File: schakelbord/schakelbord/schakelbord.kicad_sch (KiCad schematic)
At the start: 101 parts, among them J1 Rookmachine, J12 I/O nano, J15 Relais 7&8, J16 Alalog i/o, J17 Extra 1-4, J18 Extra 5-8, J19 Relais 5&6, J20 Relais 3&4, J21 Relais 1&2, J3 Power, J4 mosfets, K10 SANYOU_SRD_Form_C, K3 SANYOU_SRD_Form_C, K4 SANYOU_SRD_Form_C, K5 SANYOU_SRD_Form_C, K6 SANYOU_SRD_Form_C, K7 SANYOU_SRD_Form_C, K8 SANYOU_SRD_Form_C, K9 SANYOU_SRD_Form_C, Q1 BC337, Q10 BC337, Q11 BC337, Q12 BC337, Q13 BC337, Q14 BC337, Q15 IRLZ44N, Q2 IRLZ44N, Q3 IRLZ44N, Q5 BC337, Q6 BC337, Q9 BC337, U1 MCP23017x-x-SP

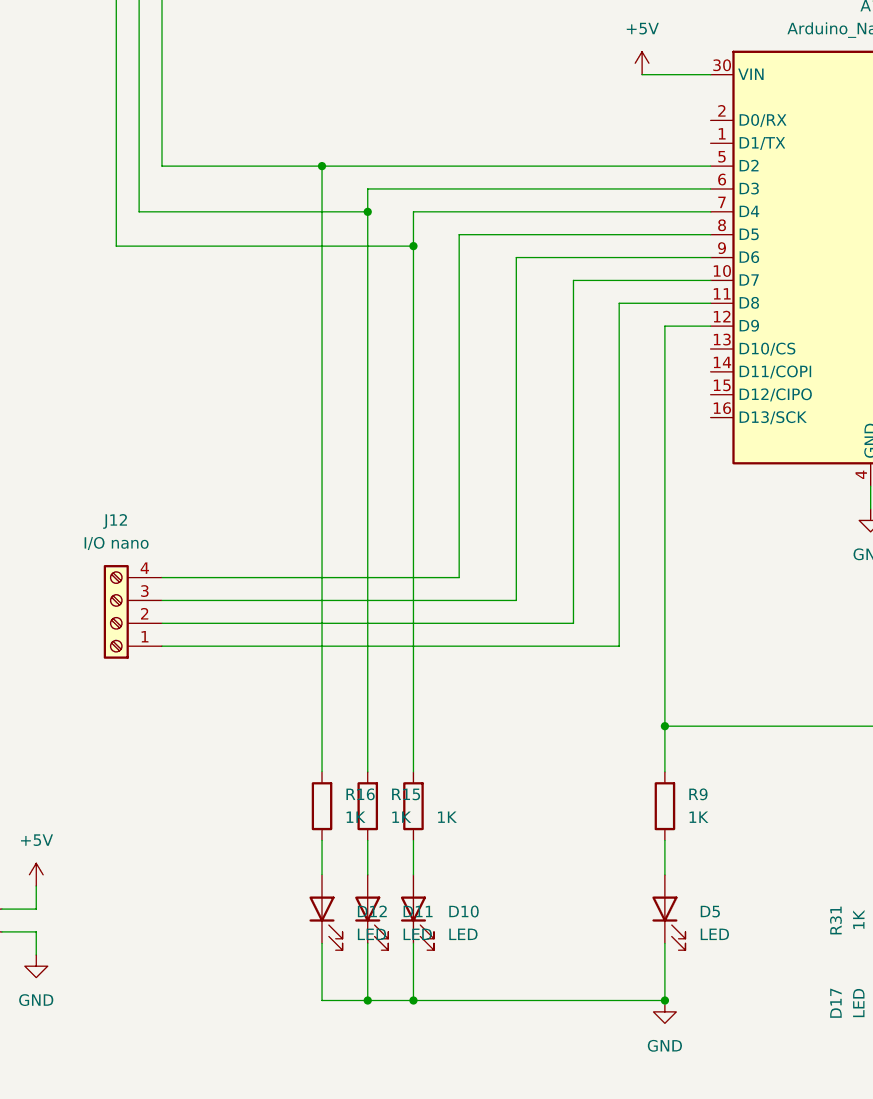
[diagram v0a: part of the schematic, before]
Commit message: pcb update
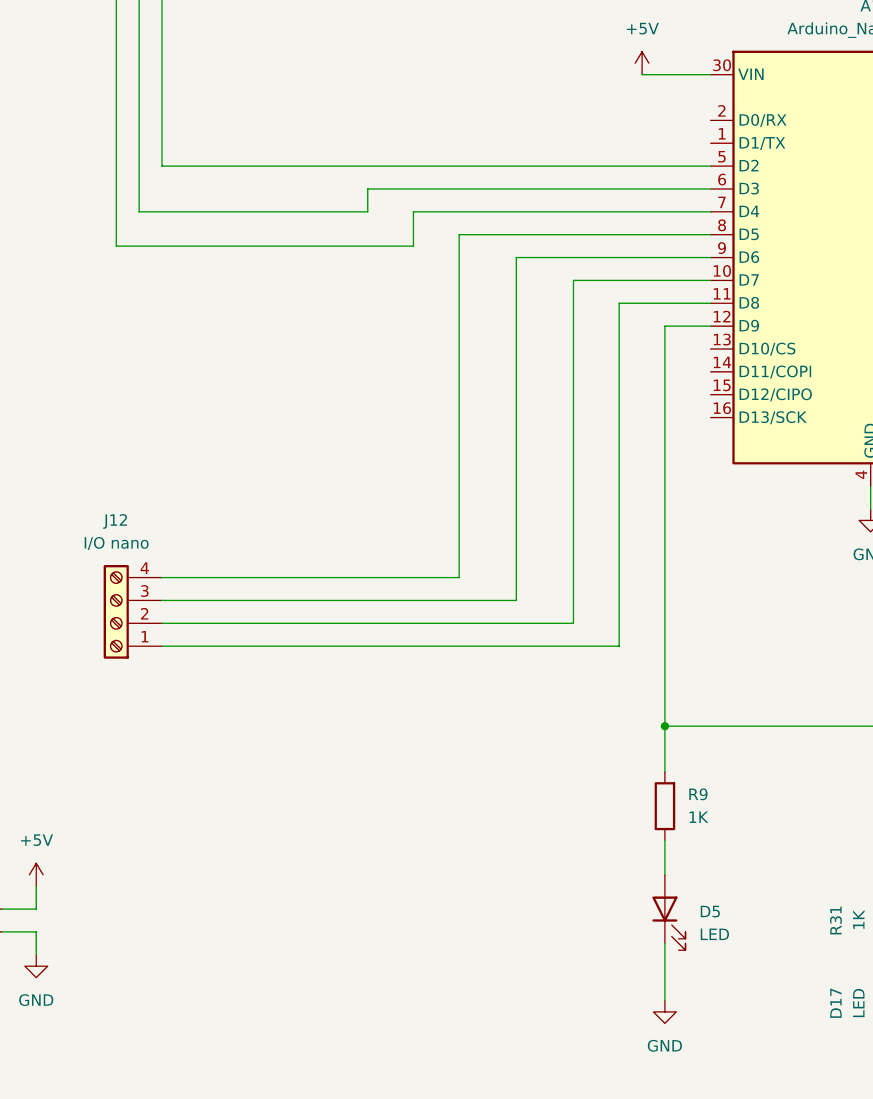
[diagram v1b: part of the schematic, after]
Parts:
- removed D10, D11, D12: LED, LED_THT:LED_D5.0mm, symbol Device:LED
- removed R14, R15, R16: 1K, Resistor_THT:R_Axial_DIN0204_L3.6mm_D1.6mm_P7.62mm_Horizontal, symbol Device:R
